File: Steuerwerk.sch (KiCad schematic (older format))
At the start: 114 parts, among them J1 2PinTerminalBlocktg, J10 2PinTerminalBlocktg, J11 2PinTerminalBlocktg, J12 2PinTerminalBlocktg, J2 2PinTerminalBlocktg, J3 3PinTerminalBlocktg, J4 3PinTerminalBlocktg, J5 2PinTerminalBlocktg, J6 2PinTerminalBlocktg, J7 2PinTerminalBlocktg, J8 2PinTerminalBlocktg, J9 2PinTerminalBlocktg, Q1 Q_PNP_BCE, U1 74ls240, U2 74541, U3 74LS161, U4 74LS138, U5 74LS138, U6 74541, U7 74LS374, U8 74LS374

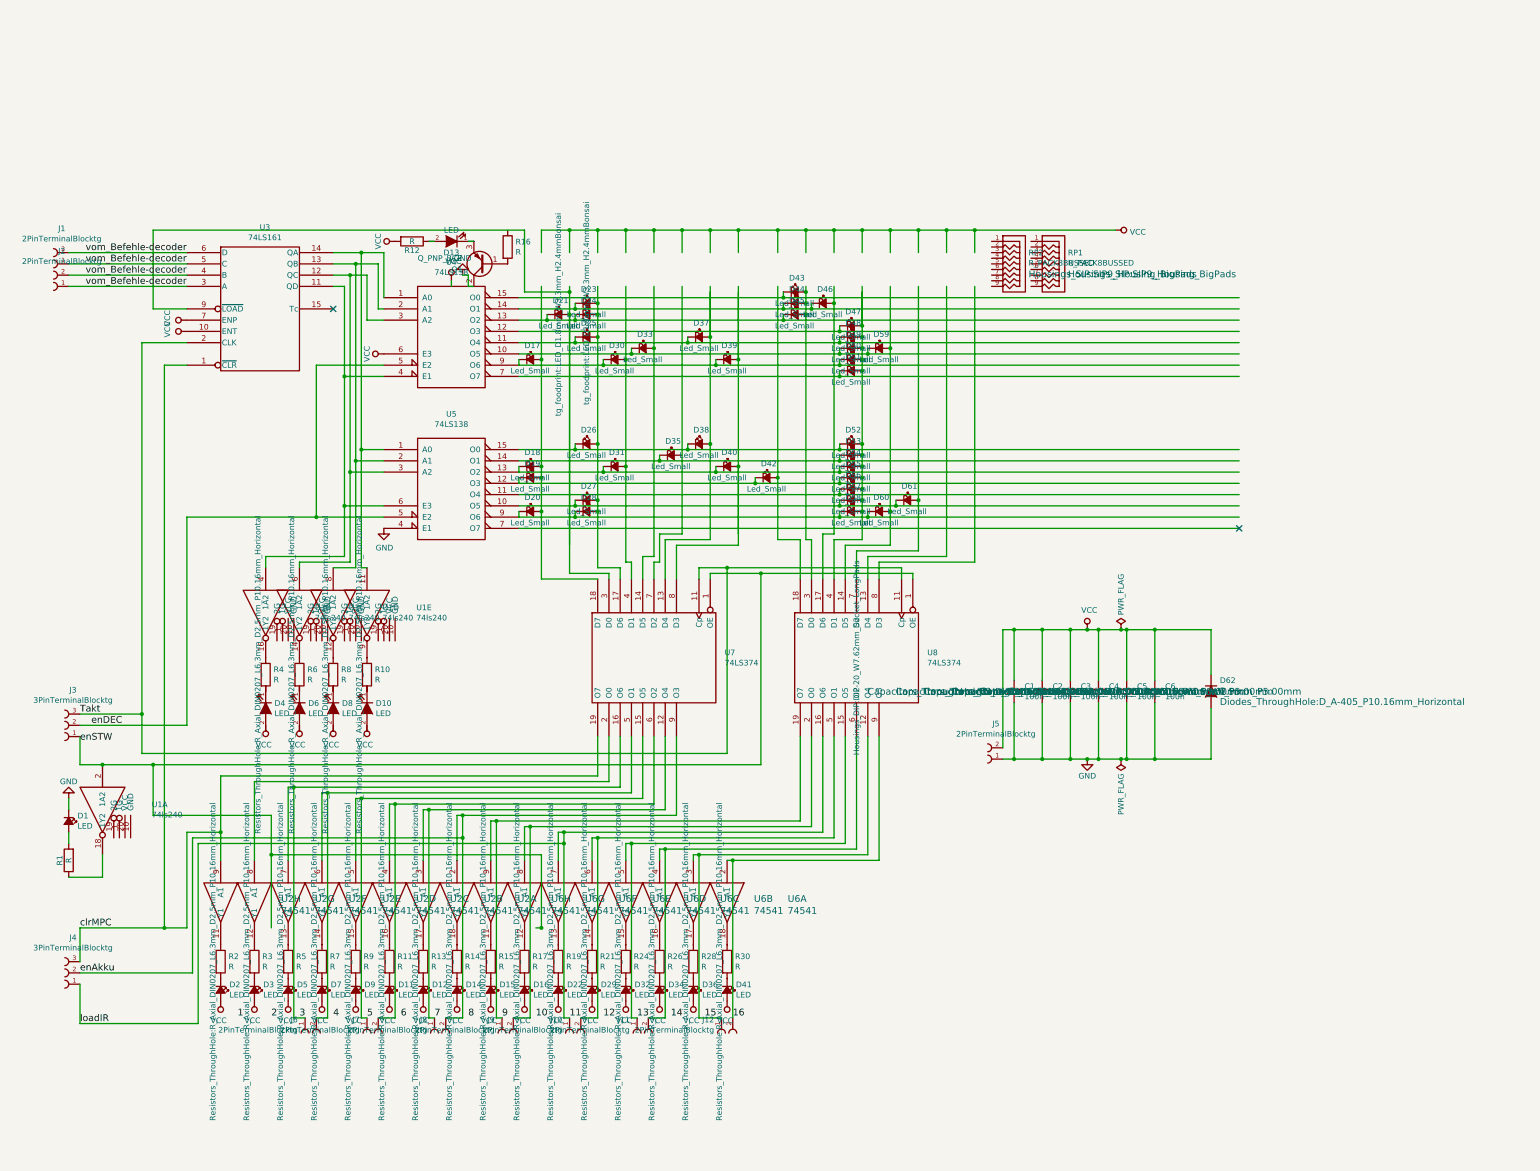
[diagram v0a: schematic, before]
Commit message: Steuerwerk: a lot of things ...
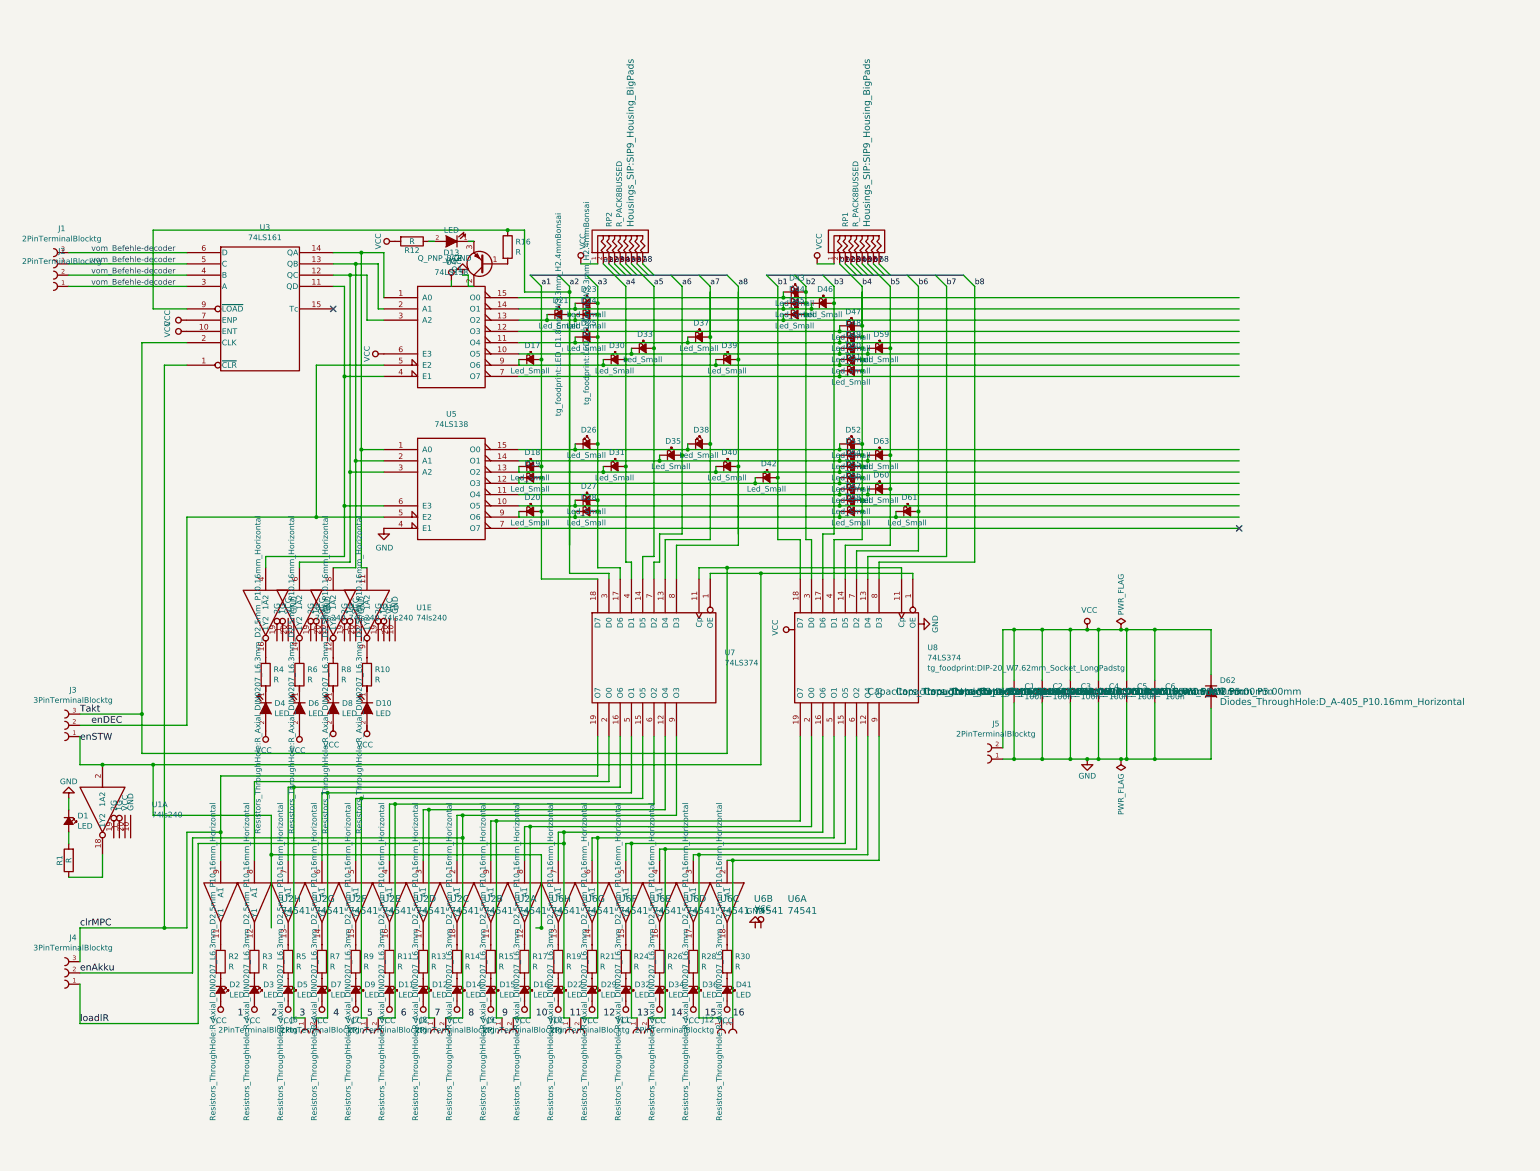
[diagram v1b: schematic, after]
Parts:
- added D63: Led_Small, tg_foodprint:LED_D1.8mm_W3.3mm_H2.4mmBonsai, symbol device:LED_Small
- U8: footprint Housings_DIP:DIP-20_W7.62mm_Socket_LongPads -> tg_foodprint:DIP-20_W7.62mm_Socket_LongPadstg
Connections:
- net labels added: a1, a2, a3, a4, a5, a6, a7, a8, b1, b2, b3, b4, b5, b6, b7, b8
- net labels removed: vom_Befehle-decoder
- wire segments 442 -> 414
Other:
- note added: "vom_Befehle-decoder"
- moved on the sheet: D60, D61, RP1, RP2

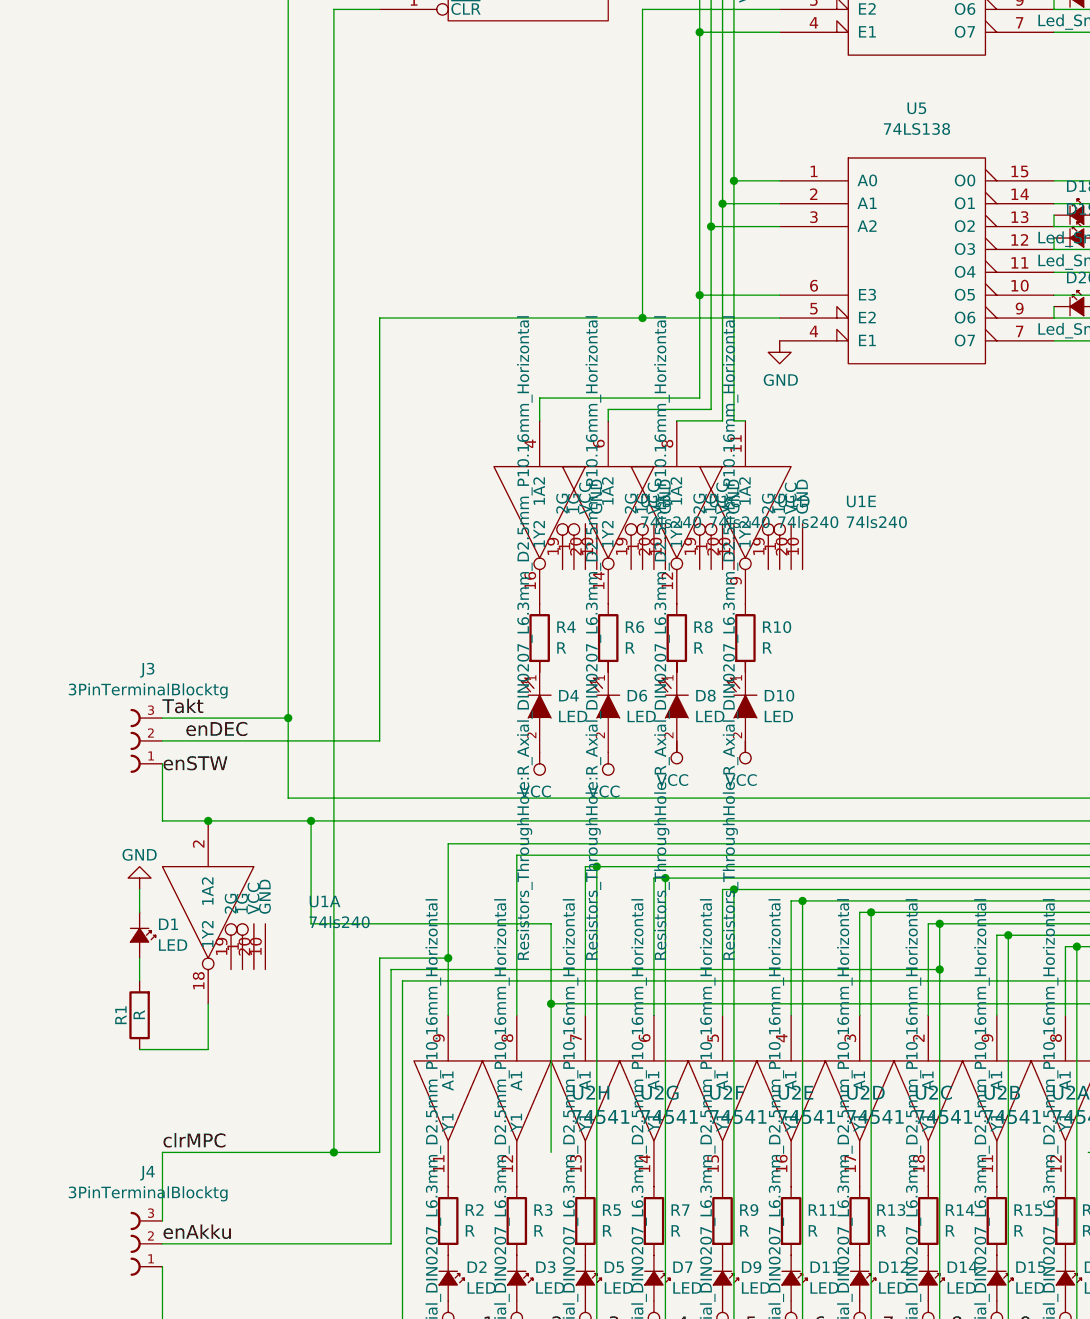
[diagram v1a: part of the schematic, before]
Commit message: steuerwerk improvements
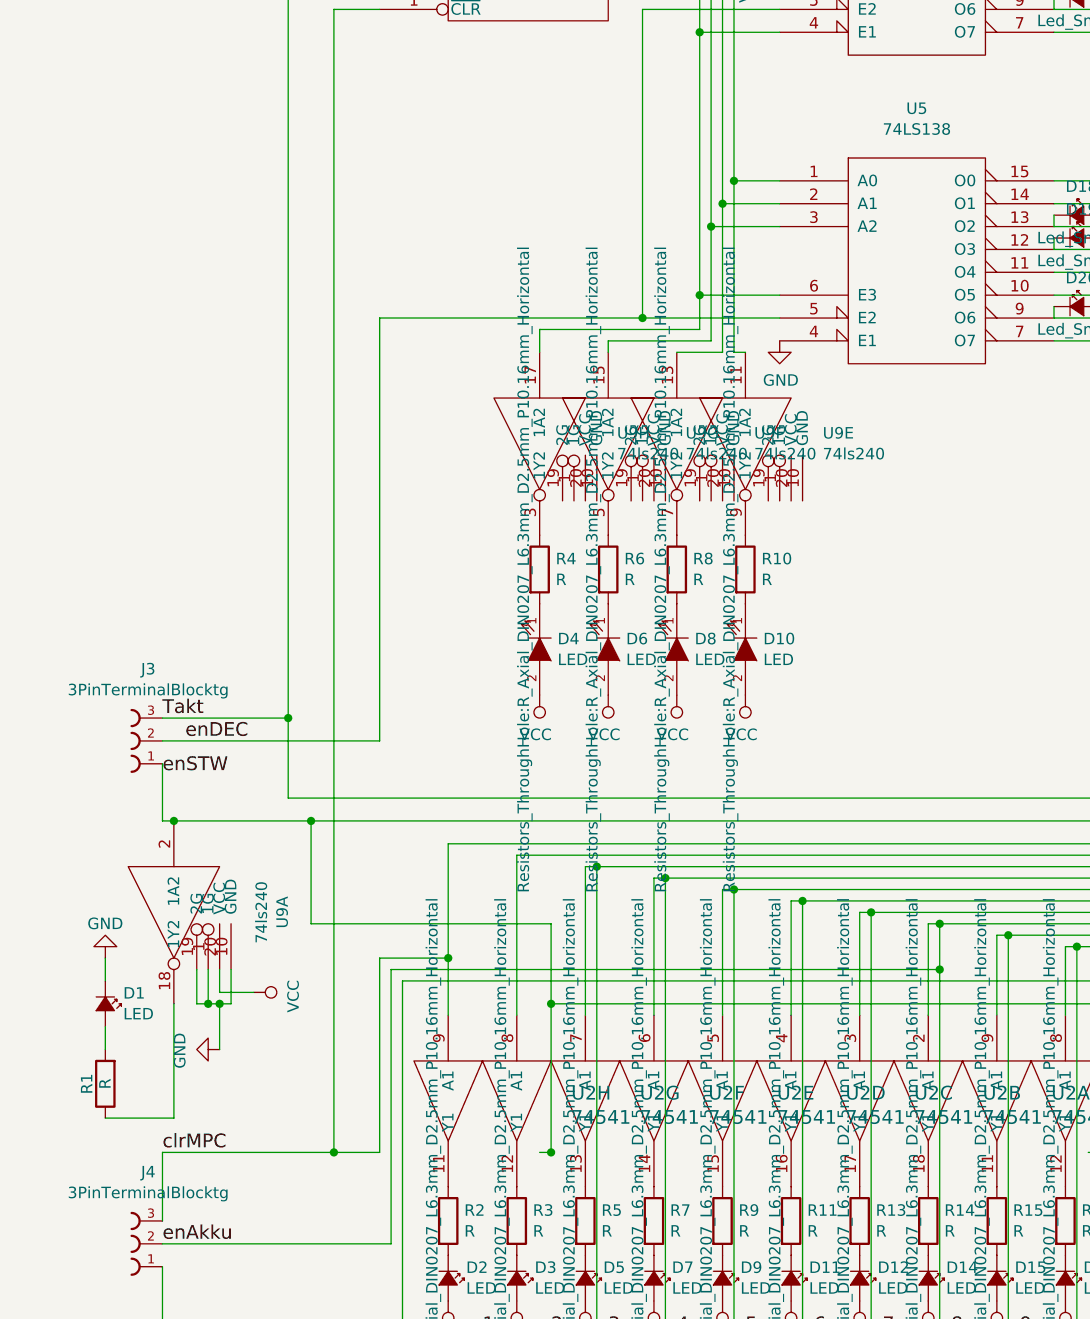
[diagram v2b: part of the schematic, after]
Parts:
- removed U1: 74ls240, Housings_DIP:DIP-20_W7.62mm_Socket_LongPads, symbol bonsai:74ls240
- added U9: 74ls240, Package_DIP:DIP-20_W7.62mm_Socket_LongPads, symbol bonsai:74ls240
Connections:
- wire segments 414 -> 424
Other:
- moved on the sheet: D1, D10, D4, D6, D8, R1, R10, R4, R6, R8

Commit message: tracs tracs tracs
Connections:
- wire segments 424 -> 422
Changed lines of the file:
@@
 Connection ~ 3200 2950
-Wire Wire Line
-	3350 1800 3550 1800
 Wire Wire Line
 	3350 700  3550 700
@@
 	3100 700  3350 700
 Connection ~ 3350 700
-Wire Wire Line
-	3350 700  3350 1800
 Connection ~ 3350 2450
-Wire Wire Line
-	3350 1800 3350 2450
-Wire Wire Line
-	3200 1000 3200 1800
-Wire Wire Line
-	3200 1800 3200 2950
-Connection ~ 3200 1800
-Wire Wire Line
-	3350 1800 3200 1800
 Connection ~ 1600 6700
 Wire Wire Line
@@
 Wire Wire Line
 	2500 6700 2550 6700
+Connection ~ 2550 6700
+Wire Wire Line
+	3200 1000 3200 1800
+Wire Wire Line
+	3350 700  3350 2450
+Wire Wire Line
+	3550 1800 3200 1800
 Wire Bus Line
 	4850 900  6600 900
 Wire Bus Line
 	6950 900  8700 900
-Connection ~ 2550 6700
+Connection ~ 3200 1800
+Wire Wire Line
+	3200 1800 3200 2950
 $EndSCHEMATC
